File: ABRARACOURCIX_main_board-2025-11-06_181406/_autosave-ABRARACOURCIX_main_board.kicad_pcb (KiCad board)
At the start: 2 copper layers, 140 x 140 mm, 72 parts, among them J1 Conn_01x02_Pin, J10 Conn_01x03_Socket, J11 Conn_01x03_Socket, J12 Conn_01x02_Pin, J2 XT60PW-M, J3 XT60PW-M, J4 Conn_01x06_Socket, J5 Conn_01x05_Socket, J6 Conn_01x03_Socket, J7 XT60PW-F, J8 Conn_01x03_Socket, J9 Conn_01x03_Socket, K1 Relai_T9GV1L14-5, Q2 NTR4101PT1G, Q3 MMBT3904, U2 Current_sens_ACS712ELCTR-20A-T, U3 AZ1117CH-3.3TRG1, U5 BNO055, U6 LMC6482, U7 LMC6482, U9 STM32F429VETx, Y2 ABS07-32.768KHZ-T

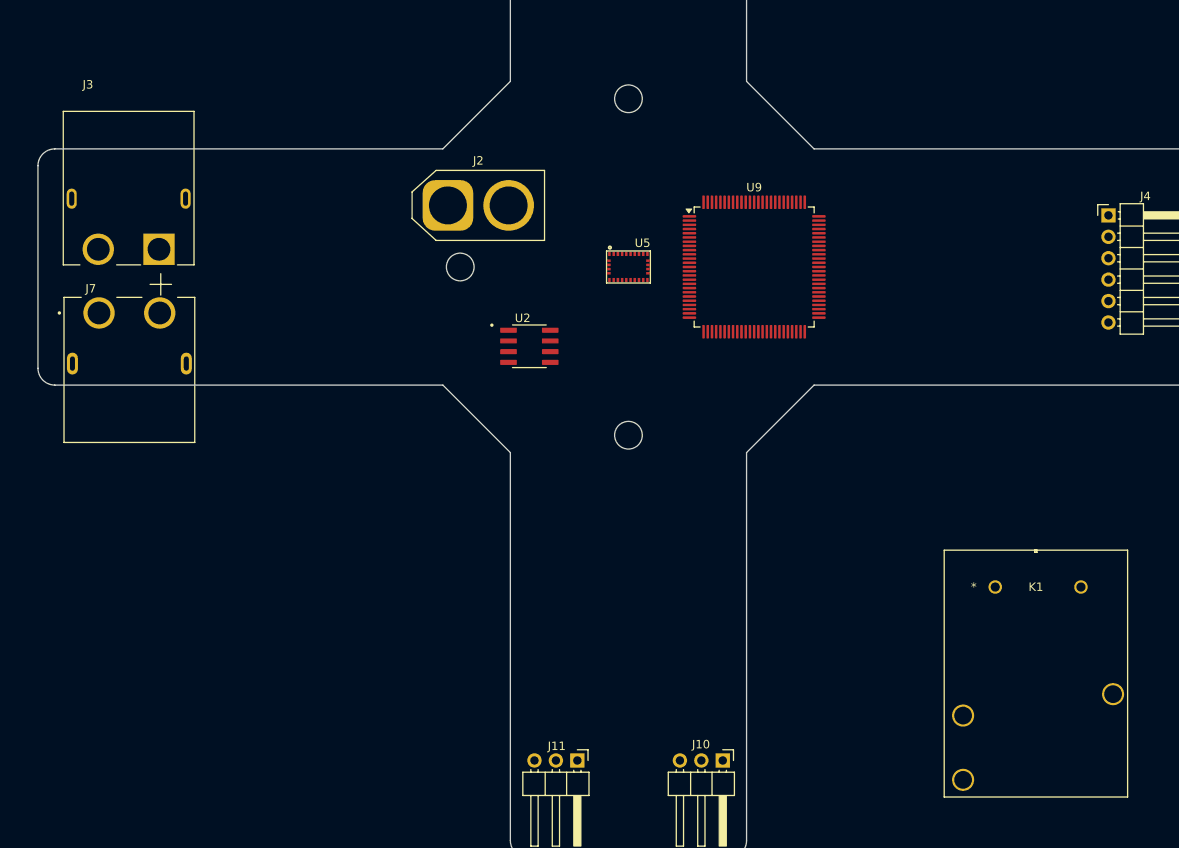
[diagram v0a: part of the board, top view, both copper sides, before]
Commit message: Modifs au circuit d'alim
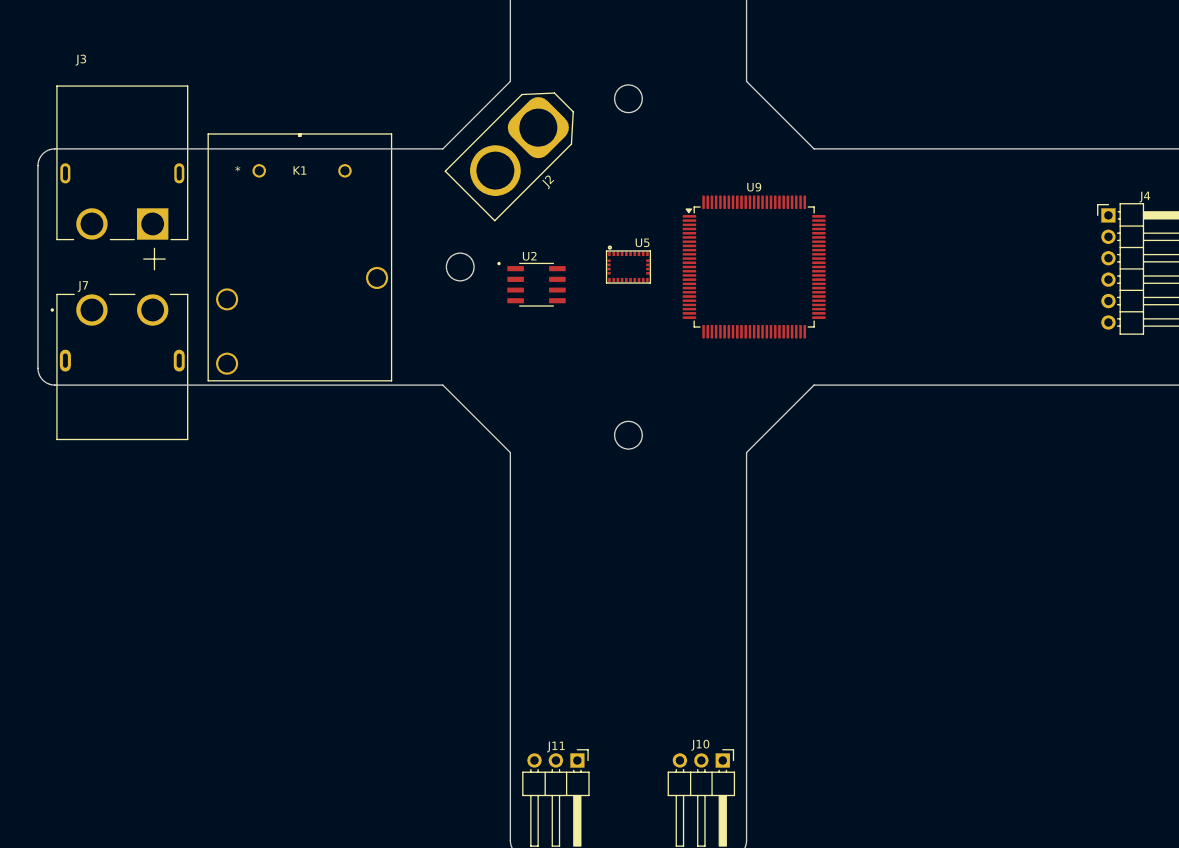
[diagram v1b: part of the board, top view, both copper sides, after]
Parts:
- moved K1 100.2 mm to (-43.8, -11.4)
- moved J2 14.1 mm to (-10.7, -16.5), turned to -135 degrees
- moved U2 7.35 mm to (-10.9, 2.10)
- moved J3 3.09 mm to (-60.0, -11.1)
- moved J7 0.91 mm to (-60.0, 5.10)
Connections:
- J3 pad S1: (no net) -> GND
- J3 pad S2: (no net) -> GND
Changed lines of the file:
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@@
 	(footprint "Librairie_footprint:Current_sens_SOIC127P600X175-8N"
 		(layer "F.Cu")
-		(at -11.745 9.4)
+		(at -10.9 2.1)
 		(property "Reference" "U2"
 			(at -0.795 -3.337 0)
@@
 	(footprint "Librairie_footprint:Relai_30A_T9GV1L14-5_TEC"
 		(layer "F.Cu")
-		(at 43.48 37.936622)
+		(at -43.77 -11.399977)
 		(tags "T9GV1L14-5 ")
 		(property "Reference" "K1"
@@
 	(footprint "Librairie_footprint:AMASS_XT60PW-M"
 		(layer "F.Cu")
-		(at -59.25 -8.1)
+		(at -60 -11.1)
 		(property "Reference" "J3"
 			(at -4.8236 -13.51498 0)
@@
 			(layers "*.Cu" "*.Mask")
 			(remove_unused_layers no)
+			(net 5 "GND")
 			(solder_mask_margin 0.102)
 		)
@@
 			(layers "*.Cu" "*.Mask")
 			(remove_unused_layers no)
+			(net 5 "GND")
 			(solder_mask_margin 0.102)
 		)
@@
 	(footprint "Connector_AMASS:AMASS_XT60-F_1x02_P7.20mm_Vertical"
 		(layer "F.Cu")
-		(at -21.4 -7.3)
+		(at -10.682144 -16.517857 -135)
 		(descr "AMASS female XT60, through hole, vertical, https://www.tme.eu/Document/2d152ced3b7a446066e6c419d84bb460/XT60%20SPEC.pdf")
 		(tags "XT60 female vertical")
 		(property "Reference" "J2"
-			(at 3.6 -5.3 180)
+			(at 3.599999 -5.3 45)
 			(layer "F.SilkS")
 			(effects
@@
 		)
 		(property "Value" "XT60PW-M"
-			(at 3.6 5.4 0)
+			(at 3.6 5.4 45)
 			(layer "F.Fab")
 			(effects
@@
 		)
 		(property "Datasheet" ""
-			(at 0 0 0)
+			(at 0 0 225)
 			(unlocked yes)
 			(layer "F.Fab")
@@
 		)
 		(property "Description" ""
-			(at 0 0 0)
+			(at 0 0 225)
 			(unlocked yes)
 			(layer "F.Fab")
@@
 		)
 		(property "MF" "AMASS"
-			(at 0 0 0)
+			(at 0 0 225)
 			(unlocked yes)
 			(layer "F.Fab")
@@
 		)
 		(property "MAXIMUM_PACKAGE_HEIGHT" "8.4 mm"
-			(at 0 0 0)
+			(at 0 0 225)
 			(unlocked yes)
 			(layer "F.Fab")
@@
 		)
 		(property "Package" "Package"
-			(at 0 0 0)
+			(at 0 0 225)
 			(unlocked yes)
 			(layer "F.Fab")
@@
 		)
 		(property "Price" "None"
-			(at 0 0 0)
+			(at 0 0 225)
 			(unlocked yes)
 			(layer "F.Fab")
@@
 		)
 		(property "Check_prices" "https://www.snapeda.com/parts/XT60PW-M/AMASS/view-part/?ref=eda"
-			(at 0 0 0)
+			(at 0 0 225)
 			(unlocked yes)
 			(layer "F.Fab")
@@
 		)
 		(property "STANDARD" "Manufacturer recommendations"
-			(at 0 0 0)
+			(at 0 0 225)
 			(unlocked yes)
 			(layer "F.Fab")
@@
 		)
 		(property "PARTREV" "V1.2"
-			(at 0 0 0)
+			(at 0 0 225)
 			(unlocked yes)
 			(layer "F.Fab")
@@
 		)
 		(property "SnapEDA_Link" "https://www.snapeda.com/parts/XT60PW-M/AMASS/view-part/?ref=snap"
-			(at 0 0 0)
+			(at 0 0 225)
 			(unlocked yes)
 			(layer "F.Fab")
@@
 		)
 		(property "MP" "XT60PW-M"
-			(at 0 0 0)
+			(at 0 0 225)
 			(unlocked yes)
 			(layer "F.Fab")
@@
 		)
 		(property "Description_1" "Socket, DC supply, male, PIN: 2"
-			(at 0 0 0)
+			(at 0 0 225)
 			(unlocked yes)
 			(layer "F.Fab")
@@
 		)
 		(property "Availability" "Not in stock"
-			(at 0 0 0)
+			(at 0 0 225)
 			(unlocked yes)
 			(layer "F.Fab")
@@
 		)
 		(property "MANUFACTURER" "AMASS"
-			(at 0 0 0)
+			(at 0 0 225)
 			(unlocked yes)
 			(layer "F.Fab")
@@
 		(attr through_hole)
 		(fp_line
-			(start -4.25 -1.6)
-			(end -4.25 1.55)
+			(start 11.450001 4.15)
+			(end 11.450001 -4.15)
 			(stroke
 				(width 0.12)
@@
 		)
 		(fp_line
-			(start -4.25 1.55)
-			(end -1.4 4.15)
+			(start 11.450001 -4.15)
+			(end -1.4 -4.150001)
 			(stroke
 				(width 0.12)
@@
 		)
 		(fp_line
-			(start -1.4 -4.15)
-			(end -4.25 -1.6)
+			(start -1.4 4.150001)
+			(end 11.450001 4.15)
 			(stroke
 				(width 0.12)
@@
 		)
 		(fp_line
-			(start -1.4 4.15)
-			(end 11.45 4.15)
+			(start -4.25 1.55)
+			(end -1.4 4.150001)
 			(stroke
 				(width 0.12)
@@
 		)
 		(fp_line
-			(start 11.45 -4.15)
-			(end -1.4 -4.15)
+			(start -1.4 -4.150001)
+			(end -4.25 -1.6)
 			(stroke
 				(width 0.12)
@@
 		)
 		(fp_line
-			(start 11.45 4.15)
-			(end 11.45 -4.15)
+			(start -4.25 -1.6)
+			(end -4.25 1.55)
 			(stroke
 				(width 0.12)
@@
 		)
 		(fp_line
-			(start -4.65 -1.85)
-			(end -1.6 -4.6)
+			(start 11.85 4.6)
+			(end -1.6 4.6)
 			(stroke
 				(width 0.05)
@@
 		)
 		(fp_line
-			(start -4.65 1.85)
-			(end -4.65 -1.85)
+			(start 11.85 -4.6)
+			(end 11.85 4.6)
 			(stroke
 				(width 0.05)
@@
 		)
 		(fp_line
-			(start -1.6 -4.6)
-			(end 11.85 -4.6)
+			(start -1.6 4.6)
+			(end -4.65 1.85)
 			(stroke
 				(width 0.05)
@@
 		)
 		(fp_line
-			(start -1.6 4.6)
-			(end -4.65 1.85)
+			(start -4.65 1.85)
+			(end -4.65 -1.85)
 			(stroke
 				(width 0.05)
@@
 		)
 		(fp_line
-			(start 11.85 -4.6)
-			(end 11.85 4.6)
+			(start -1.6 -4.6)
+			(end 11.85 -4.6)
 			(stroke
 				(width 0.05)
@@
 		)
 		(fp_line
-			(start 11.85 4.6)
-			(end -1.6 4.6)
+			(start -4.65 -1.85)
+			(end -1.6 -4.6)
 			(stroke
 				(width 0.05)
@@
 		)
 		(fp_line
-			(start -4.15 -1.55)
-			(end -4.15 1.55)
+			(start 11.35 4.049999)
+			(end 11.35 -4.049999)
 			(stroke
 				(width 0.12)
@@
 		)
 		(fp_line
-			(start -4.15 1.55)
-			(end -1.4 4.05)
+			(start 11.35 -4.049999)
+			(end -1.4 -4.05)
 			(stroke
 				(width 0.12)
@@
 		)
 		(fp_line
-			(start -1.4 -4.05)
-			(end -4.15 -1.55)
+			(start -1.4 4.05)
+			(end 11.35 4.049999)
 			(stroke
 				(width 0.12)
@@
 		)
 		(fp_line
-			(start -1.4 4.05)
-			(end 11.35 4.05)
+			(start -4.150001 1.55)
+			(end -1.4 4.05)
 			(stroke
 				(width 0.12)
@@
 		)
 		(fp_line
-			(start 11.35 -4.05)
-			(end -1.4 -4.05)
+			(start -1.4 -4.05)
+			(end -4.150001 -1.55)
 			(stroke
 				(width 0.12)
@@
 		)
 		(fp_line
-			(start 11.35 4.05)
-			(end 11.35 -4.05)
+			(start -4.150001 -1.55)
+			(end -4.150001 1.55)
 			(stroke
 				(width 0.12)
@@
 		)
 		(fp_text user "${REFERENCE}"
-			(at 3.6 0.05 0)
+			(at 3.6 0.05 45)
 			(layer "F.Fab")
 			(effects
@@
 		)
 		(pad "1" thru_hole roundrect
-			(at 0 0)
+			(at 0 0 225)
 			(size 6 6)
 			(drill 4.5)
@@
 		)
 		(pad "2" thru_hole circle
-			(at 7.2 0)
+			(at 7.2 0 225)
 			(size 6 6)
 			(drill 4.5)
@@
 	(footprint "Librairie_footprint:AMASS_XT60PW-F"
 		(layer "F.Cu")
-		(at -59.1625 5.45)
+		(at -60 5.1)
 		(property "Reference" "J7"
 			(at -4.575 -2.885 0)
